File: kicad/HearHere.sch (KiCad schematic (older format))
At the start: 3 parts

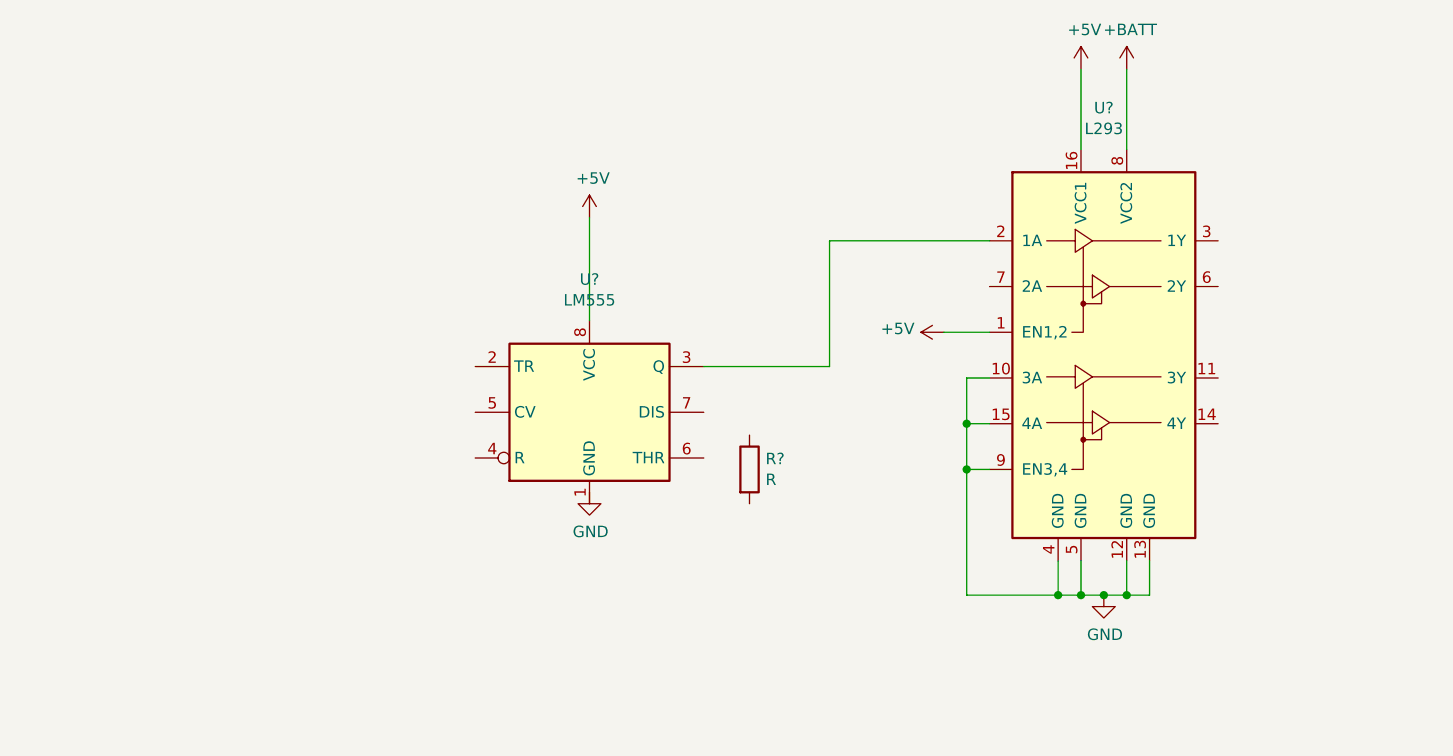
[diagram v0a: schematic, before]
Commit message: Adjusted Project Poster
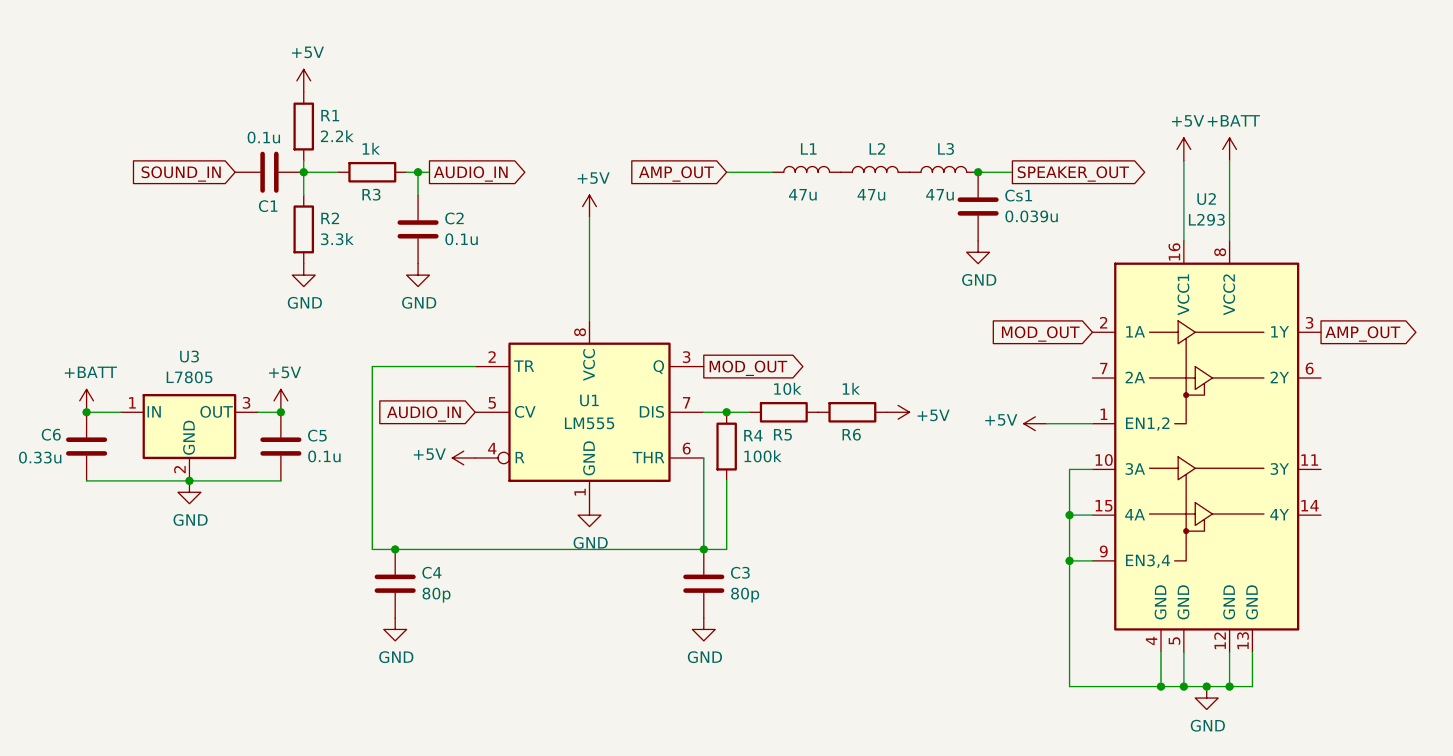
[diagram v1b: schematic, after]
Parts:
- removed R?: R, symbol Device:R
- added C1, C2, C5: 0.1u, Capacitors_THT:C_Axial_L3.8mm_D2.6mm_P7.50mm_Horizontal, symbol Device:C
- added C3, C4: 80p, Capacitors_THT:C_Axial_L3.8mm_D2.6mm_P7.50mm_Horizontal, symbol Device:C
- added C6: 0.33u, Capacitors_THT:C_Axial_L3.8mm_D2.6mm_P7.50mm_Horizontal, symbol Device:C
- added Cs1: 0.039u, Capacitors_THT:C_Axial_L3.8mm_D2.6mm_P7.50mm_Horizontal, symbol Device:C
- added L1, L2, L3: 47u, Inductors_THT:L_Axial_L9.5mm_D4.0mm_P12.70mm_Horizontal_Fastron_SMCC, symbol Device:L
- added R1: 2.2k, Resistors_THT:R_Axial_DIN0309_L9.0mm_D3.2mm_P12.70mm_Horizontal, symbol Device:R
- added R2: 3.3k, Resistors_THT:R_Axial_DIN0309_L9.0mm_D3.2mm_P12.70mm_Horizontal, symbol Device:R
- added R3: 1k, Resistors_THT:R_Axial_DIN0411_L9.9mm_D3.6mm_P12.70mm_Horizontal, symbol Device:R
- added R4: 100k, Resistors_THT:R_Axial_DIN0411_L9.9mm_D3.6mm_P12.70mm_Horizontal, symbol Device:R
- added R5: 10k, Resistors_THT:R_Axial_DIN0309_L9.0mm_D3.2mm_P12.70mm_Horizontal, symbol Device:R
- added R6: 1k, Resistors_THT:R_Axial_DIN0309_L9.0mm_D3.2mm_P12.70mm_Horizontal, symbol Device:R
- added U3: L7805, TO_SOT_Packages_THT:TO-220-3_Horizontal, symbol Regulator_Linear:L7805
- U1: renamed from U?; footprint (none) -> Housings_DIP:DIP-8_W7.62mm_Socket
- U2: renamed from U?; footprint Package_DIP:DIP-16_W7.62mm -> Housings_DIP:DIP-16_W7.62mm_Socket
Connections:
- net +5V: now also U1.4 (R), C5.1, R1.1, R6.1, U3.3 (OUT)
- net +BATT: now also C6.1, U3.1 (IN)
- net GND: now also U1.1 (GND), C2.2, C3.2, C4.2, C5.2, C6.2, Cs1.2, R2.2, U3.2 (GND)
- net at U1.2 (TR): now also U1.6 (THR), C3.1, C4.1, R4.2
- net MOD_OUT: now reaches U1.3 (Q), U2.2 (1A)
- net AUDIO_IN: now reaches U1.5 (CV)
- net AUDIO_IN: now also C2.1, R3.1
- net at U1.7 (DIS): now also R4.1, R5.2
- net AMP_OUT: now reaches U2.3 (1Y)
- net AMP_OUT: now also L1.1
- new net: L1.2, L2.1
- new net: L2.2, L3.1
- new net: R5.1, R6.2
- new net: C1.1, R1.2, R2.1, R3.2
- new net SOUND_IN: C1.2
- new net SPEAKER_OUT: Cs1.1, L3.2
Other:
- moved on the sheet: U2
